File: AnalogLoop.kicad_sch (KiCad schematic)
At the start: 24 parts, among them J18 u.fl, J19 u.fl, U5 ADA4075-2, U6 ADG419BR

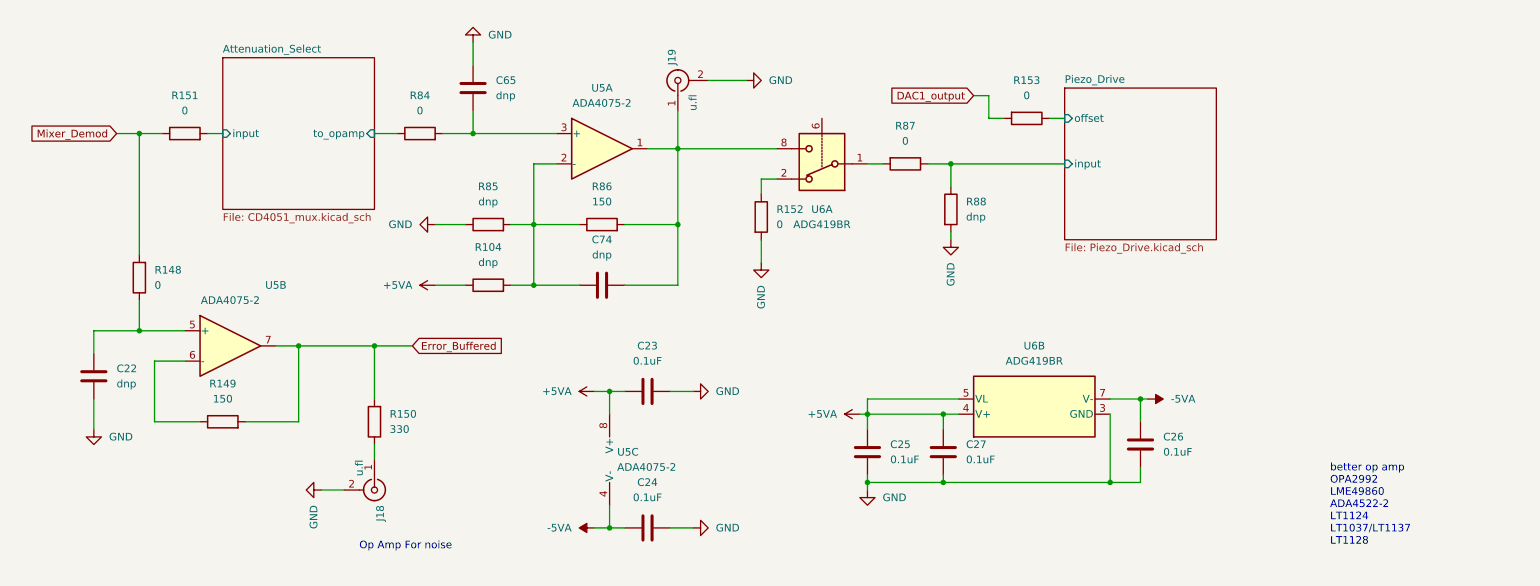
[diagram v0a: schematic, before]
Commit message: Analog section complete!
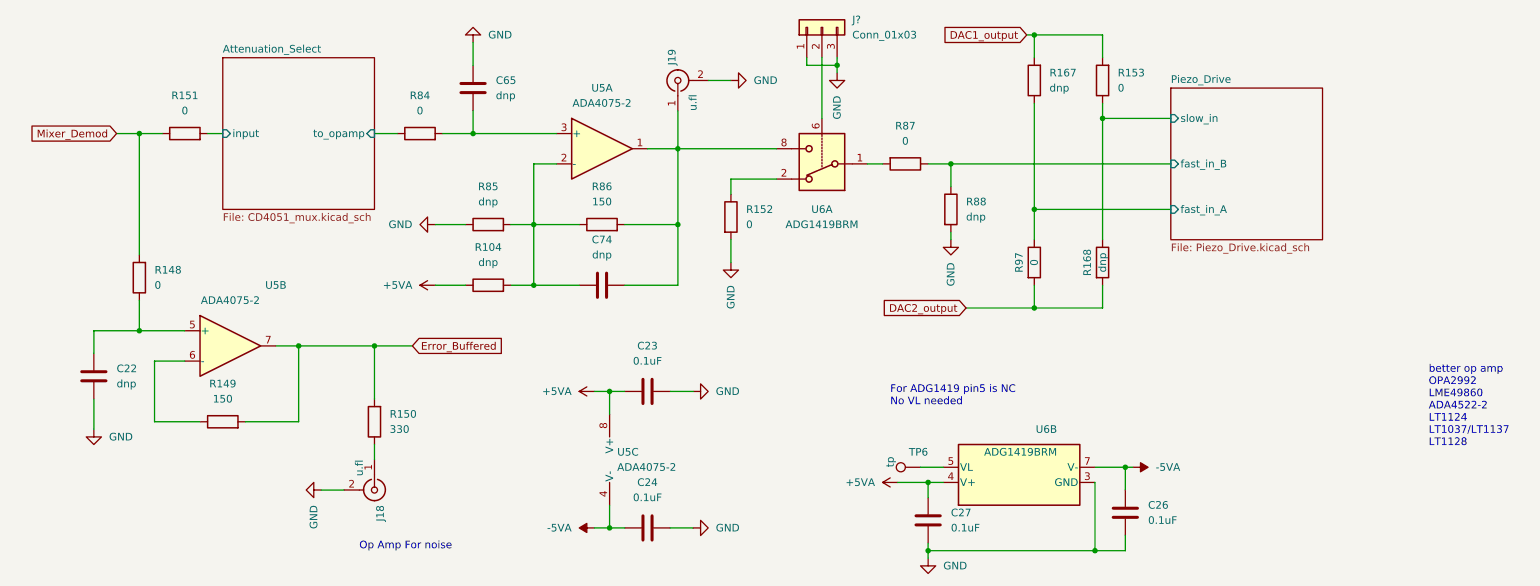
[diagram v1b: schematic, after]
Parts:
- removed C25: 0.1uF, Capacitor_SMD:C_0603_1608Metric_Pad1.08x0.95mm_HandSolder, symbol Device:C
- removed U6: ADG419BR, Package_SO:SOIC-8_3.9x4.9mm_P1.27mm, symbol Analog_Switch:ADG419BR
- added J?: Conn_01x03, Connector_PinHeader_2.54mm:PinHeader_1x03_P2.54mm_Vertical, symbol Connector_Generic:Conn_01x03
- added R167, R168: dnp, Resistor_SMD:R_0805_2012Metric, symbol Device:R
- added R97: 0, Resistor_SMD:R_0805_2012Metric, symbol Device:R
- added TP6: tp, TestPoint:TestPoint_Pad_D1.0mm, symbol Connector:TestPoint
- added U6: ADG1419BRM, Package_SO:MSOP-8_3x3mm_P0.65mm, symbol Analog_Switch:ADG419BRM
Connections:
- net +5VA: now also U6.4 (V+)
- net -5VA: now also U6.7 (V-)
- net DAC1_output: now also R167.2
- net GND: now also J?.1 (Pin_1), J?.3 (Pin_3), U6.3 (GND)
- net at R87.2: now also U6.1
- net at R152.1: now also U6.2
- net at C74.2, J19.1 (In), R86.2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: now also U6.8
- net Piezo_Drive/input renamed Piezo_Drive/fast_in_B
- net Piezo_Drive/offset renamed Piezo_Drive/slow_in
- net Piezo_Drive/slow_in: now also R168.1
- new net: J?.2 (Pin_2), U6.6
- new net: TP6.1, U6.5 (VL)
- new net DAC2_output: R168.2, R97.2
- new net Piezo_Drive/fast_in_A: R167.1, R97.1
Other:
- sheet Piezo_Drive ports: added fast_in_A, fast_in_B, slow_in; removed input, offset
- note added: "For ADG1419 pin5 is NC No VL needed"
- moved on the sheet: C26, C27, R152, R153
